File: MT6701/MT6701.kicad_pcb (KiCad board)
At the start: 2 copper layers, 23.2 x 23.2 mm, 3 parts, among them J1 Conn_01x05_Pin, U1 MT6701QT

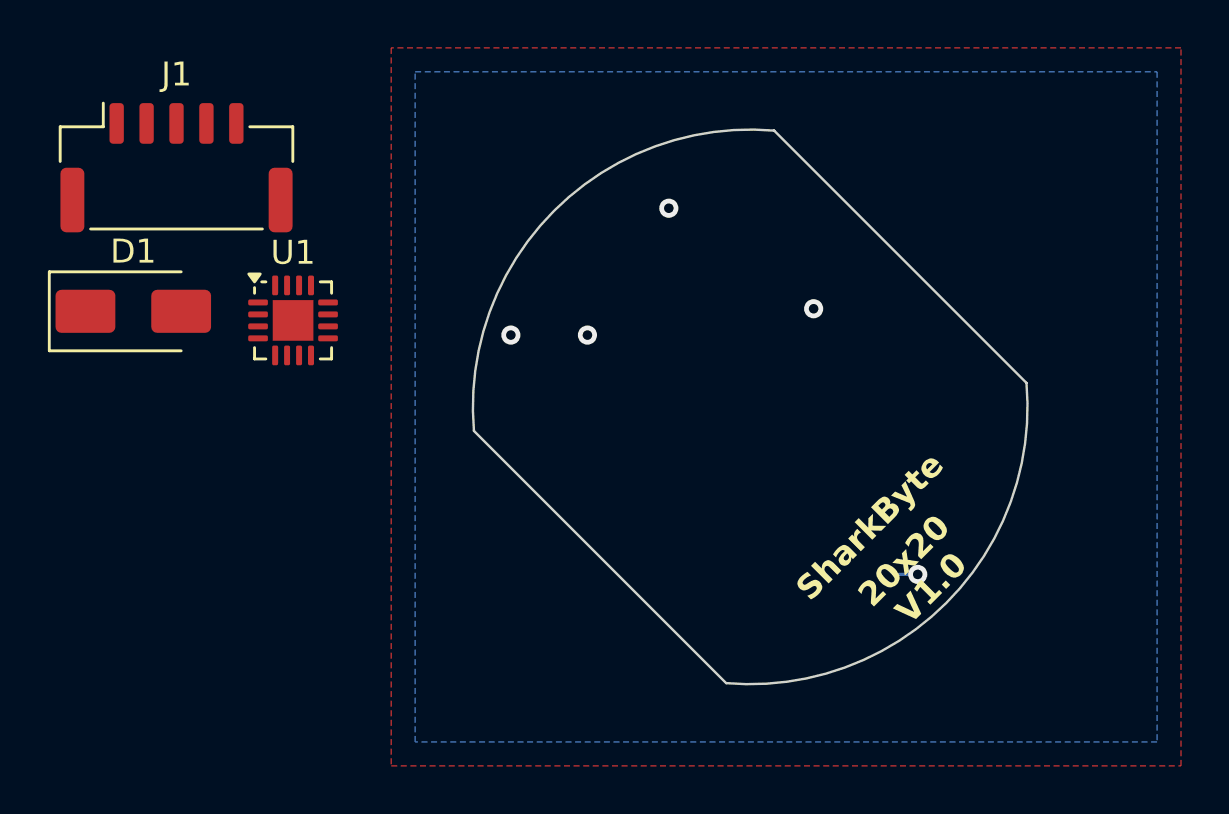
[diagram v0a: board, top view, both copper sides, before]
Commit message: V1 Order
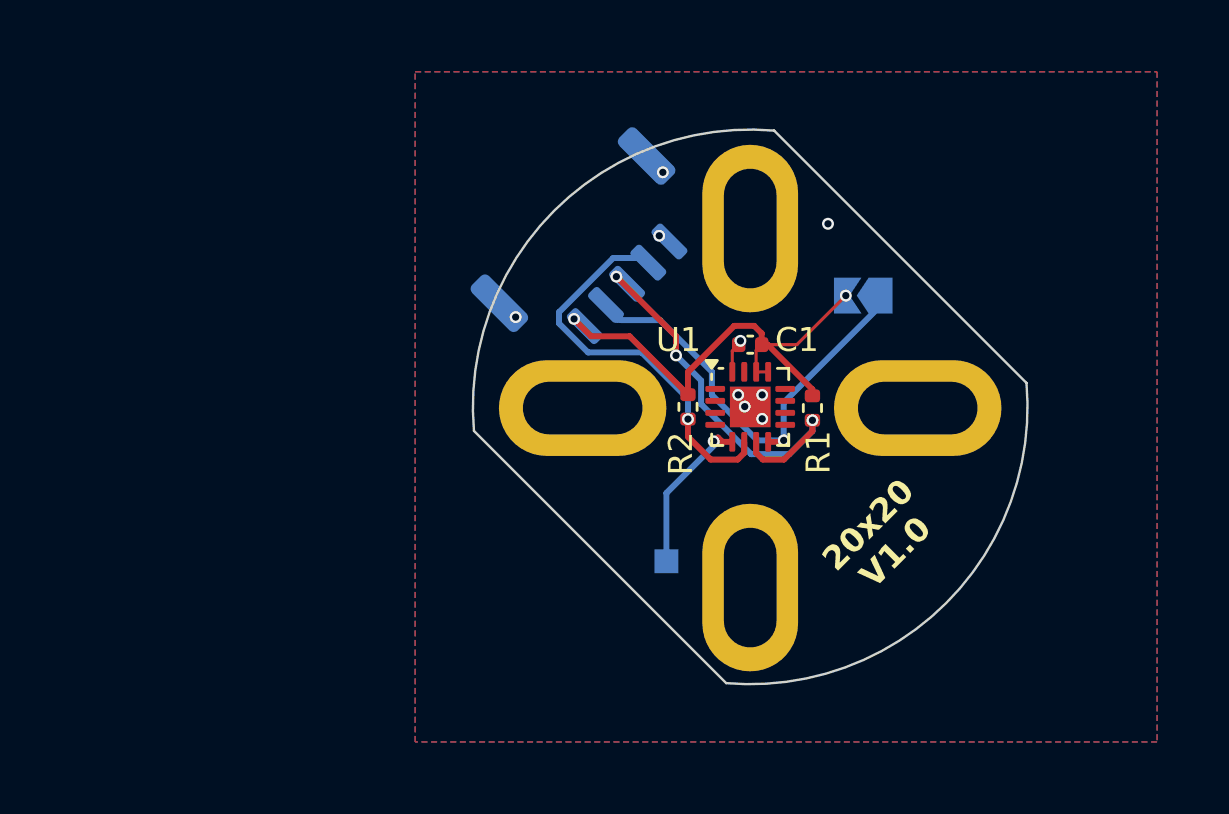
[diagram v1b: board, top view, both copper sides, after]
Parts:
- removed D1: SMAJ6.0A, Diode_SMD:D_SMA
- added C1: 100nF, Capacitor_SMD:C_0402_1005Metric, F.Cu at (150.0, 147.4)
- added G***: LOGO, Sharkbite:Logo1 8x8, B.Cu at (149.3, 150.2)
- added JP1: SolderJumper_2_Open, Jumper:SolderJumper-2_P1.3mm_Open_TrianglePad1.0x1.5mm, B.Cu at (154.7, 145.3)
- added R1: 5K, Resistor_SMD:R_0402_1005Metric, F.Cu at (152.6, 150.1)
- added R2: 5K, Resistor_SMD:R_0402_1005Metric, F.Cu at (147.4, 150.0)
- added REF**: 18XX-20XX Motor, Sharkbite:18XX-20XX Motor, F.Cu at (150.0, 150.1)
- added TP1: TestPoint, TestPoint:TestPoint_Pad_1.0x1.0mm, B.Cu at (146.5, 156.4)
- J1: moved to B.Cu
- moved U1 19.4 mm to (150.0, 150.0)
- moved J1 17.9 mm to (143.6, 143.6), turned to 45 degrees
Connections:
- J1 pad MP: (no net) -> GND
- U1 pad 15: Net-(U1-OUT) -> unconnected-(U1-OUT-Pad15)
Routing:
- net +5V: track 0.00 -> 20.8 mm, vias 0 -> 2
- net /VDD/CSN: track 0.00 -> 20.1 mm, vias 0 -> 1
- net /SCL/CLK: track 0.00 -> 17.0 mm, vias 0 -> 3
- net /SDA/DO: track 0.00 -> 16.8 mm, vias 0 -> 1
- net Net-(U1-PUSH): track 0.00 -> 6.74 mm, vias 0 -> 1
- net GND: track 0.81 -> 1.25 mm, vias 5 -> 9
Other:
- board text removed: "I2C"
- board text removed: "PWM"
